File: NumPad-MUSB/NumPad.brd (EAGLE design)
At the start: 88.9 x 142.9 mm, 174 parts, among them J1 J, J10 J, J11 J, J12 J, J13 J, J14 J, J15 J, J16 J, J17 J, J2 J, J3 J, J4 J, J5 J, J6 J, J7 J, J8 J, J9 J

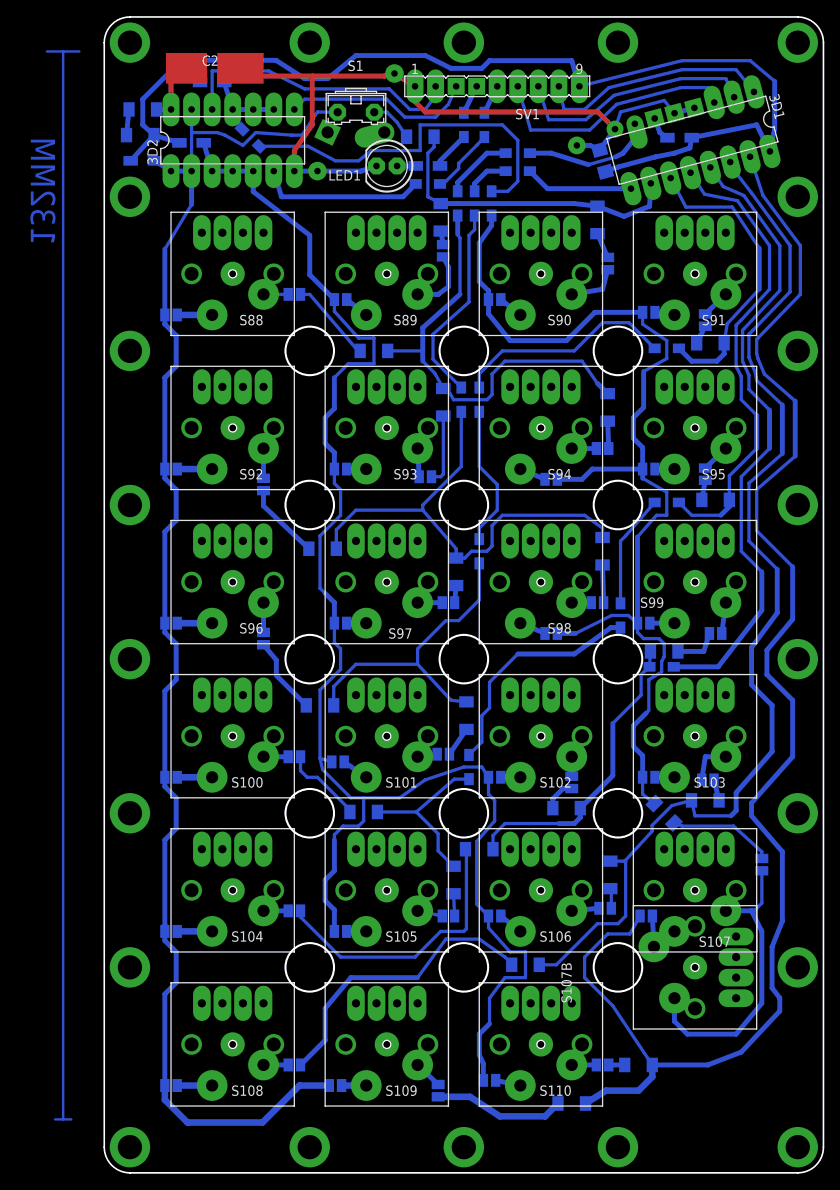
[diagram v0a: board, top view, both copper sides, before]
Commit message: + stab reserv
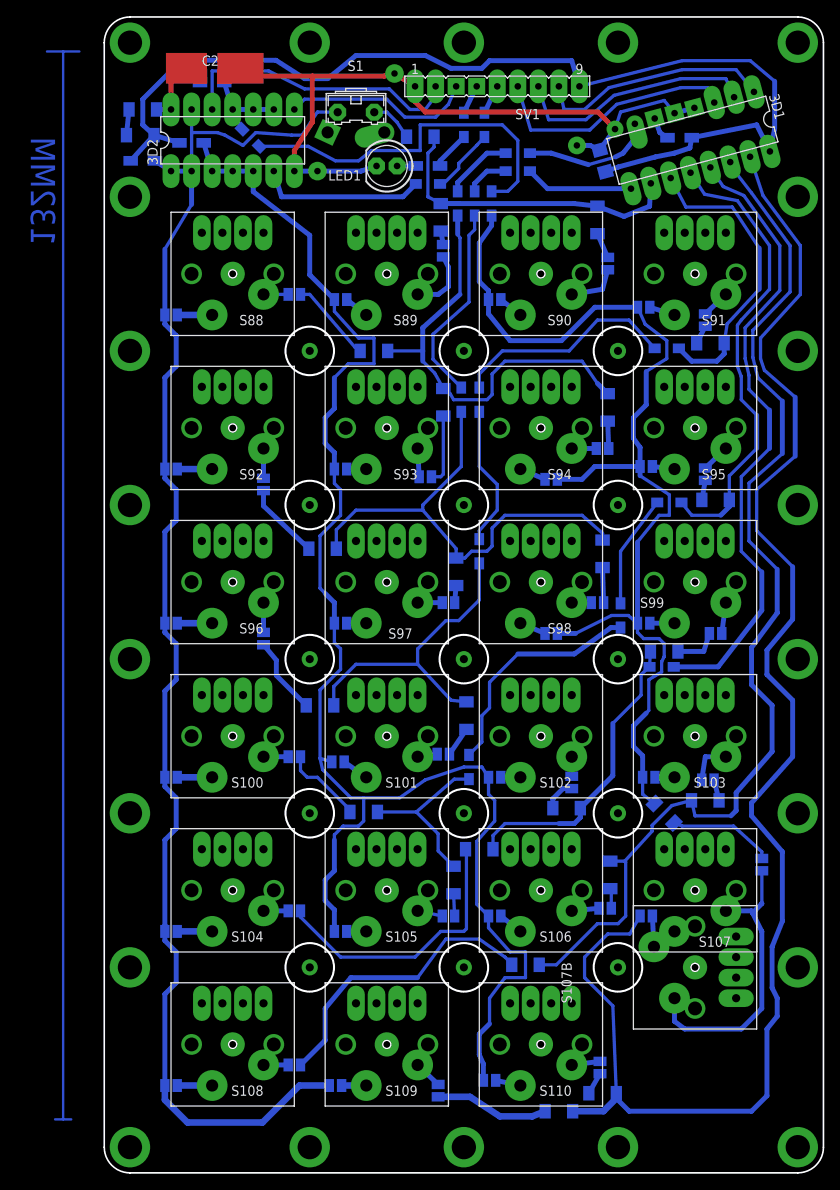
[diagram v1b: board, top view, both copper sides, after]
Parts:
- moved D110 5.65 mm to (79.7, 23.8)
- moved D109 1.85 mm to (74.3, 21.6)
- moved JA91 0.90 mm to (84.8, 121.0)
- moved JB110 0.45 mm to (79.4, 27.0), turned to 270 degrees
- moved JA95 0.45 mm to (85.1, 101.3)
- moved D98 0.32 mm to (79.7, 90.5)
- moved J3 0.32 mm to (87.9, 96.8)
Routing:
- net SCK: track 176.6 -> 186.6 mm
- net N$333: track 16.2 -> 14.1 mm
- net N$335: track 1.98 -> 2.78 mm
- net N$282: track 2.43 -> 3.19 mm
